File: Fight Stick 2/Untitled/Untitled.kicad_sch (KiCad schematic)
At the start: 18 parts, among them U1 Elite-C

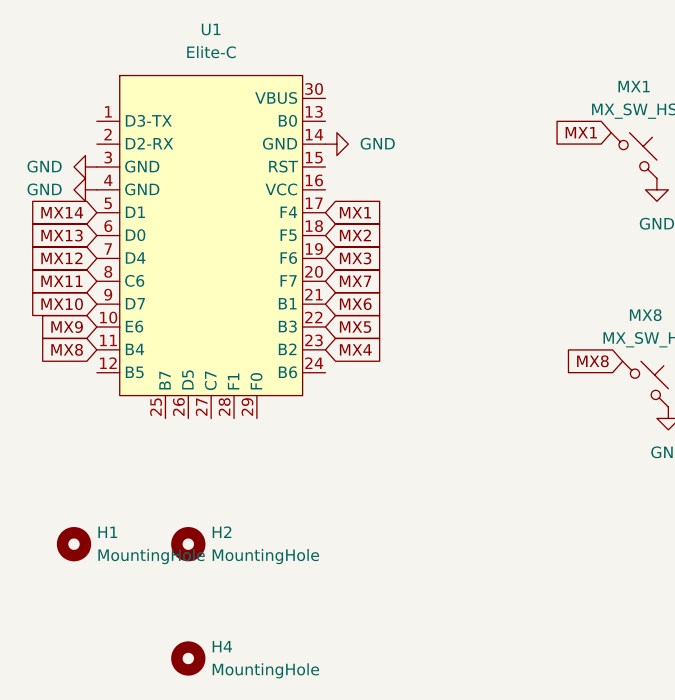
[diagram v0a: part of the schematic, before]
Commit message: second version upload
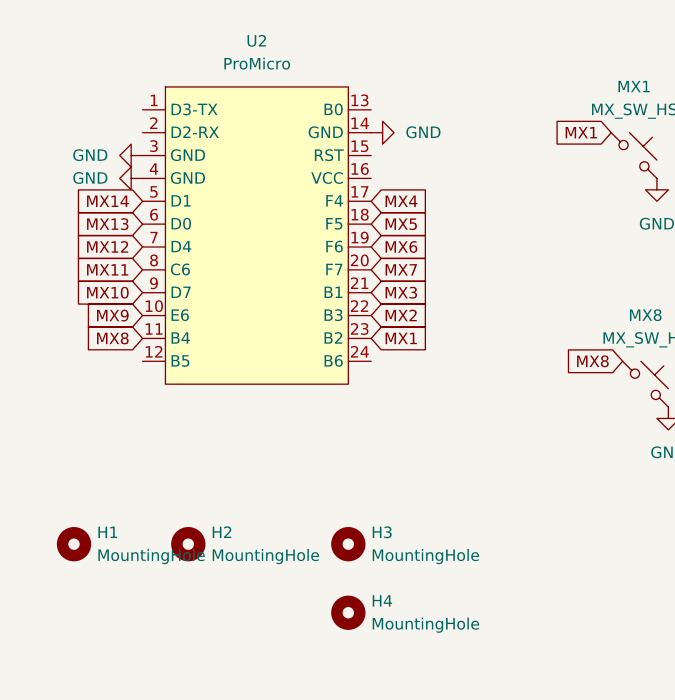
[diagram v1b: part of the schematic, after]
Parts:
- removed U1: Elite-C, Keebio-Parts.pretty-master:Elite-C-castellated-24pin-holes, symbol marbastlib-promicroish:Elite-C
- added H4: MountingHole, MountingHole:MountingHole_2.2mm_M2_DIN965_Pad, symbol Mechanical:MountingHole
- added U2: ProMicro, Fight Stick 2:ProMicro_USBdn, symbol marbastlib-promicroish:Arduino_ProMicro
- MX1, MX10, MX11, MX12, MX13, MX14, MX2, MX3, MX4, MX5, MX6, MX7, MX8, MX9: footprint keyswitches.pretty-2.1:Kailh_socket_MX_optional -> Fight Stick 2:MX_optional
- renumbered H4 to H3
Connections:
- net GND: now also U2.14 (GND), U2.3 (GND), U2.4 (GND)
- net MX1: now also U2.23 (B2)
- net MX10: now also U2.9 (D7)
- net MX11: now also U2.8 (C6)
- net MX12: now also U2.7 (D4)
- net MX13: now also U2.6 (D0)
- net MX14: now also U2.5 (D1)
- net MX2: now also U2.22 (B3)
- net MX3: now also U2.21 (B1)
- net MX4: now also U2.17 (F4)
- net MX5: now also U2.18 (F5)
- net MX6: now also U2.19 (F6)
- net MX7: now also U2.20 (F7)
- net MX8: now also U2.11 (B4)
- net MX9: now also U2.10 (E6)
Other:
- moved on the sheet: H3
